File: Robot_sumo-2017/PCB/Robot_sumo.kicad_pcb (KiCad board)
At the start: 2 copper layers, 70 x 90 mm, 63 parts, among them J1 CONN_Batt, J2 CONN_C1, J3 CONN_C3, J4 CONN_C2, J5 CONN_C4, J6 CONN_M1, J7 CONN_M2, J8 CONN_distance, U1 Arduino-nano, U2 LM324, U3 NE555, U4 L293, U5 trou-3, U6 trou-3, U7 trou-3

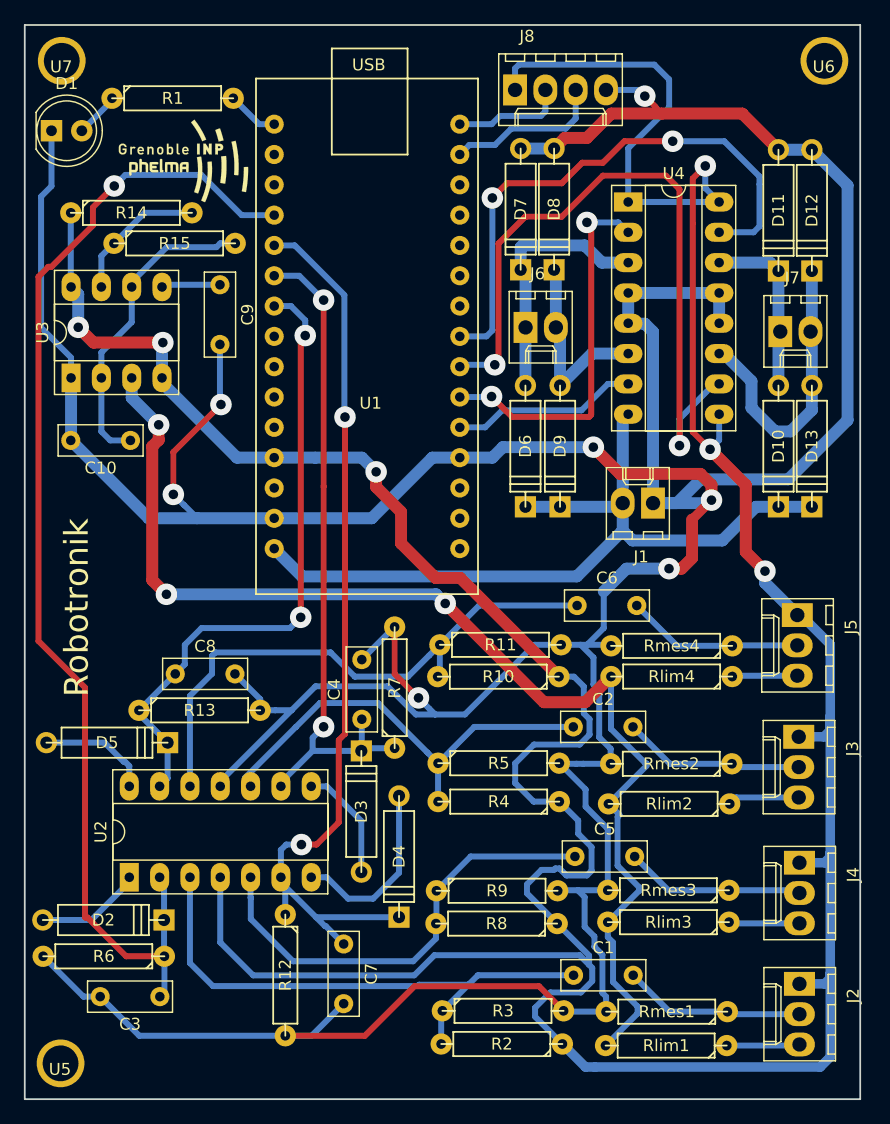
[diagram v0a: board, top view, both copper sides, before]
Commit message: plan de masse
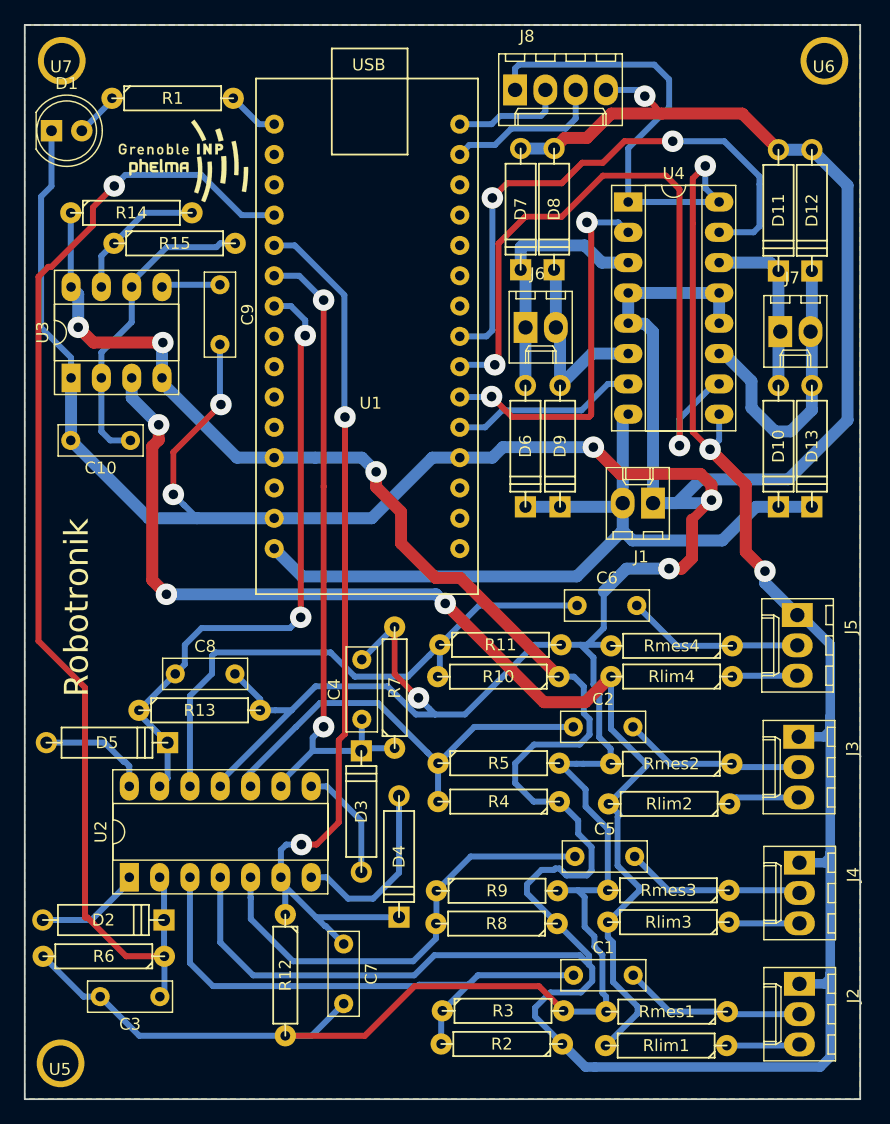
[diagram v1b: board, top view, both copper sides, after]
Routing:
- added copper zone on B.Cu, net GND
- added copper zone on F.Cu, net GND
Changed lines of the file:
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@@
   (general
     (links 128)
-    (no_connects 2)
+    (no_connects 0)
     (area 104.924999 89.855 175.595 180.075001)
     (thickness 1.6)
@@
   (segment (start 119.014484 105.73545) (end 115.034484 105.73545) (width 0.5) (layer B.Cu) (net 54))
   (segment (start 115.034484 105.73545) (end 112.474484 108.29545) (width 0.5) (layer B.Cu) (net 54))
+  (zone (net 1) (net_name GND) (layer B.Cu) (hatch edge 0.508)
+    (connect_pads (clearance 1))
+    (min_thickness 0.4)
+    (fill yes (arc_segments 16) (thermal_gap 0.508) (thermal_bridge_width 0.508))
+    (polygon
+      (pts
+        (xy 105 180) (xy 105 90) (xy 175 90) (xy 175 180)
+      )
+    )
+  )
+  (zone (net 1) (net_name GND) (layer F.Cu) (hatch edge 0.508)
+    (connect_pads (clearance 1))
+    (min_thickness 0.4)
+    (fill yes (arc_segments 16) (thermal_gap 0.508) (thermal_bridge_width 0.508))
+    (polygon
+      (pts
+        (xy 105 180) (xy 105 90) (xy 175 90) (xy 175 180)
+      )
+    )
+  )
 )
